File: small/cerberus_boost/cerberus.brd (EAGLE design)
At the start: 33 x 80 mm, 31 parts, among them Q1 2N5088, Q2 2N5088, Q3 2N5087

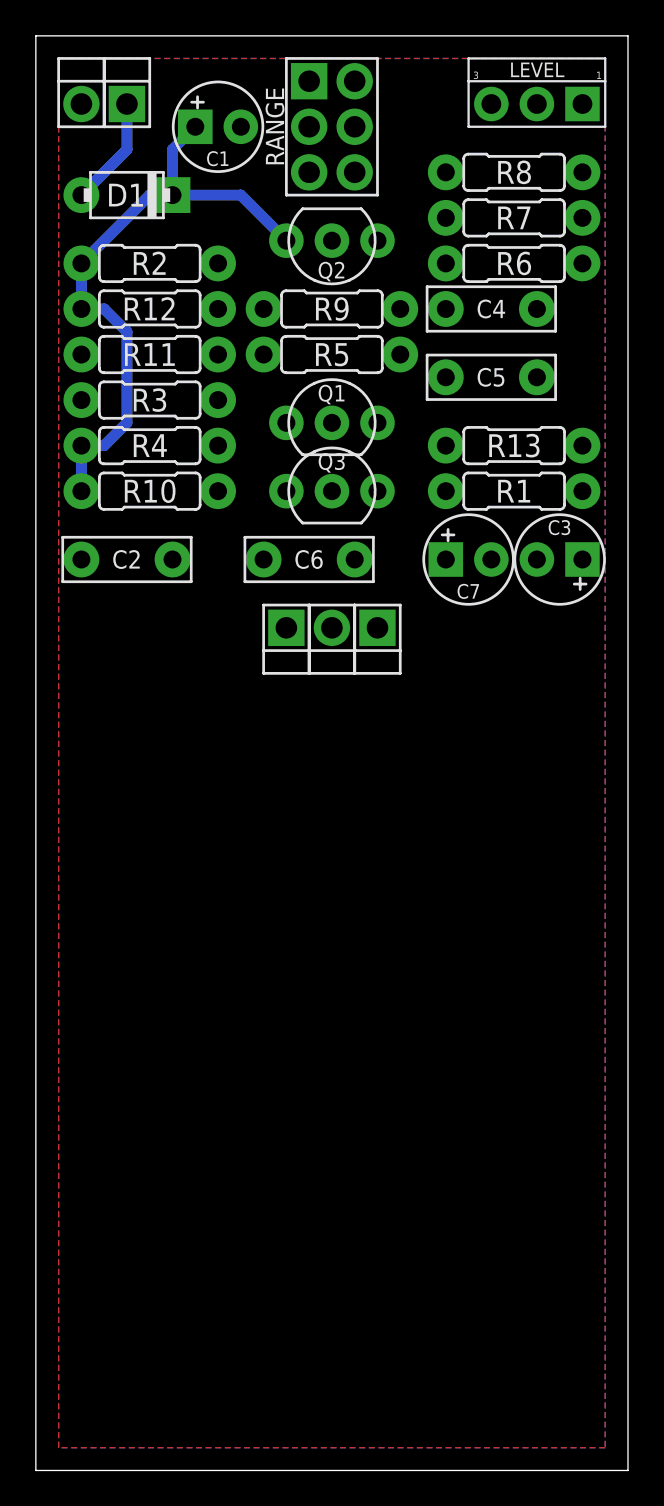
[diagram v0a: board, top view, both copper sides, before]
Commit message: formatting updates
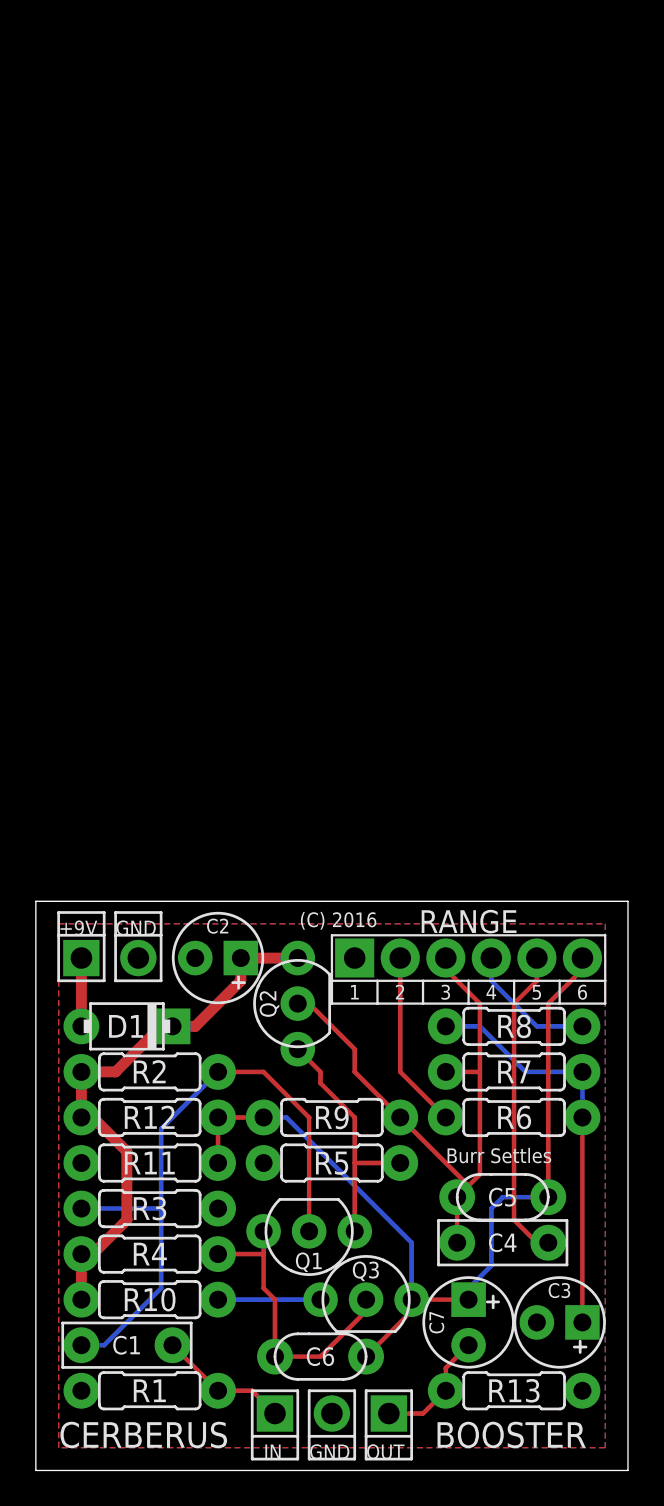
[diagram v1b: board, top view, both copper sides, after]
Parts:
- removed LEVEL: 10kA, potentiometers:PADS_SMALL
- C1: value 100u -> 47n; device capacitors-elec:050_020_1 -> capacitors-film:BOX_SMALL
- C2: value 47n -> 100u; device capacitors-film:BOX_SMALL -> capacitors-elec:050_020_1
- C5, C6: device capacitors-film:BOX_SMALL -> capacitors-film:050X030_025_2
- RANGE: device switches:DPDT -> switches:DPDT_PADS
- moved C1 68.1 mm to (5.08, 6.99)
- moved R1 54.1 mm to (6.35, 4.45), turned to 0 degrees
- moved R13 52.7 mm to (26.7, 4.45)
- moved C4 52.1 mm to (26.0, 12.7), turned to 180 degrees
- moved PAD3 47.7 mm to (5.71, 28.6)
- moved PAD1 47.7 mm to (2.54, 28.6)
- moved R6 47.6 mm to (26.7, 19.7), turned to 0 degrees
- moved R8 47.6 mm to (26.7, 24.8)
- moved R7 47.6 mm to (26.7, 22.2)
- moved RANGE 47.0 mm to (24.1, 28.6)
- moved D1 46.4 mm to (5.08, 24.8)
- moved C5 45.7 mm to (26.0, 15.2), turned to 180 degrees
- moved Q3 45.1 mm to (18.4, 9.53)
- moved Q1 45.1 mm to (15.2, 13.3), turned to 180 degrees
- moved R10 45.1 mm to (6.35, 9.53)
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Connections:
- removed net N$3: C7.-, LEVEL.3, R13.2
- net GND: now also C2.-; no longer C1.-, LEVEL.1
- net IN: now also C1.2; no longer C2.2
- net N$1: now also C1.1; no longer C2.1
- net N$10: now also RANGE.P$3; no longer RANGE.A3
- net N$14: now also RANGE.P$4; no longer RANGE.B1
- net N$6: now also RANGE.P$6; no longer RANGE.B3
- net N$7: now also C2.+; no longer C1.+
- net N$8: now also RANGE.P$2; no longer RANGE.A2
- net N$9: now also RANGE.P$5; no longer RANGE.B2
- net OUT: now also C7.-, R13.2; no longer LEVEL.2
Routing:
- net N$6: track 0.00 -> 50.0 mm
- net N$1: track 0.00 -> 36.1 mm
- net N$10: track 0.00 -> 33.6 mm
- net N$12: track 0.00 -> 22.6 mm
- net N$9: track 0.00 -> 17.6 mm
- net N$4: track 0.00 -> 16.6 mm
- net N$5: track 0.00 -> 14.0 mm
- net N$8: track 0.00 -> 9.94 mm
- net N$14: track 0.00 -> 7.40 mm
- net IN: track 0.00 -> 7.29 mm
- net OUT: track 0.00 -> 6.77 mm
- net N$2: track 0.00 -> 5.71 mm
- net N$7: track 34.7 -> 31.0 mm
- net +9V: track 6.13 -> 3.81 mm
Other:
- board size 33 x 80 mm -> 33 x 31.7 mm
- board text added: "(C) 2016"
- board text added: "+9V"
- board text added: "BOOSTER"
- board text added: "Burr Settles"
- board text added: "CERBERUS"
- board text added: "GND"
- board text added: "IN"
- board text added: "OUT"
